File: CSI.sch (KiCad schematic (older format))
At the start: 19 parts

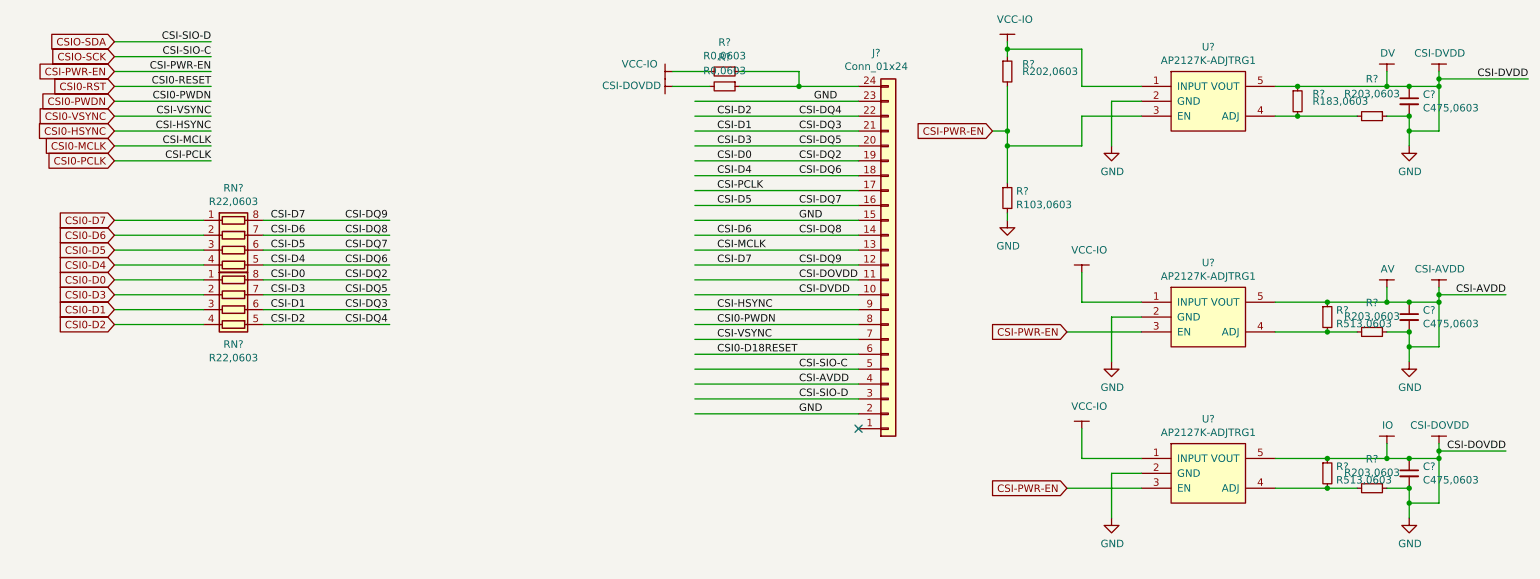
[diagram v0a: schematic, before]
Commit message: update,
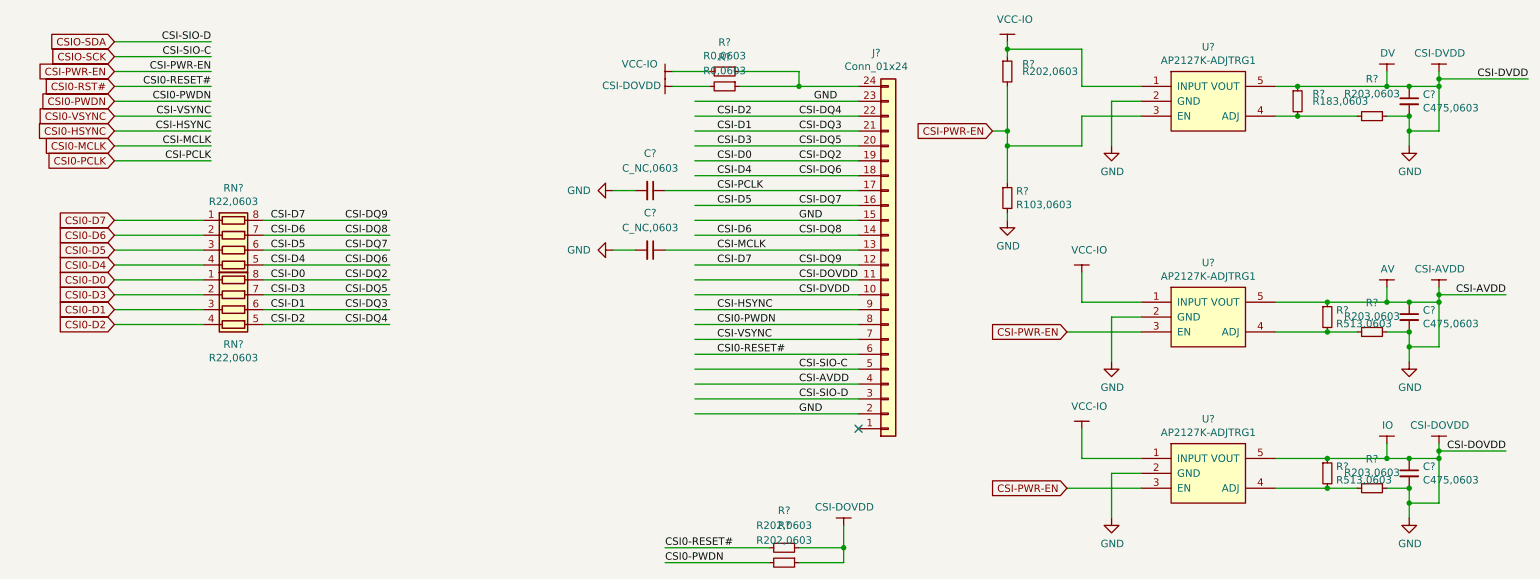
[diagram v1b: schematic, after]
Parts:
- added C? (x2): C_NC,0603, Capacitor_SMD:C_0603_1608Metric_Pad1.05x0.95mm_HandSolder, symbol taobao-components:C_NC,0603
- added R? (x2): R202,0603, Resistor_SMD:R_0603_1608Metric_Pad1.05x0.95mm_HandSolder, symbol taobao-r:R202,0603
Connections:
- net labels added: CSI0-RESET#, CSI0-RST#
- net labels removed: CSI0-D18RESET, CSI0-RESET, CSI0-RST
- wire segments 123 -> 131
